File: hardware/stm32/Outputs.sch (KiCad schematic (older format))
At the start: 34 parts, among them J10 Screw_Terminal_01x02, J11 Screw_Terminal_01x02, J12 Screw_Terminal_01x02, J13 Screw_Terminal_01x02, J6 Screw_Terminal_01x02, J7 Conn_01x02, J8 Screw_Terminal_01x02, J9 Screw_Terminal_01x02, Q1 Q_NMOS_GSD, Q2 Q_NMOS_GSD, Q3 Q_NMOS_GSD, Q4 Q_NMOS_GSD, Q5 Q_NMOS_GSD, Q6 Q_NMOS_GSD, U10 PC817, U11 PC817, U5 PC817, U6 PC817, U7 PC817, U8 PC817, U9 PC817

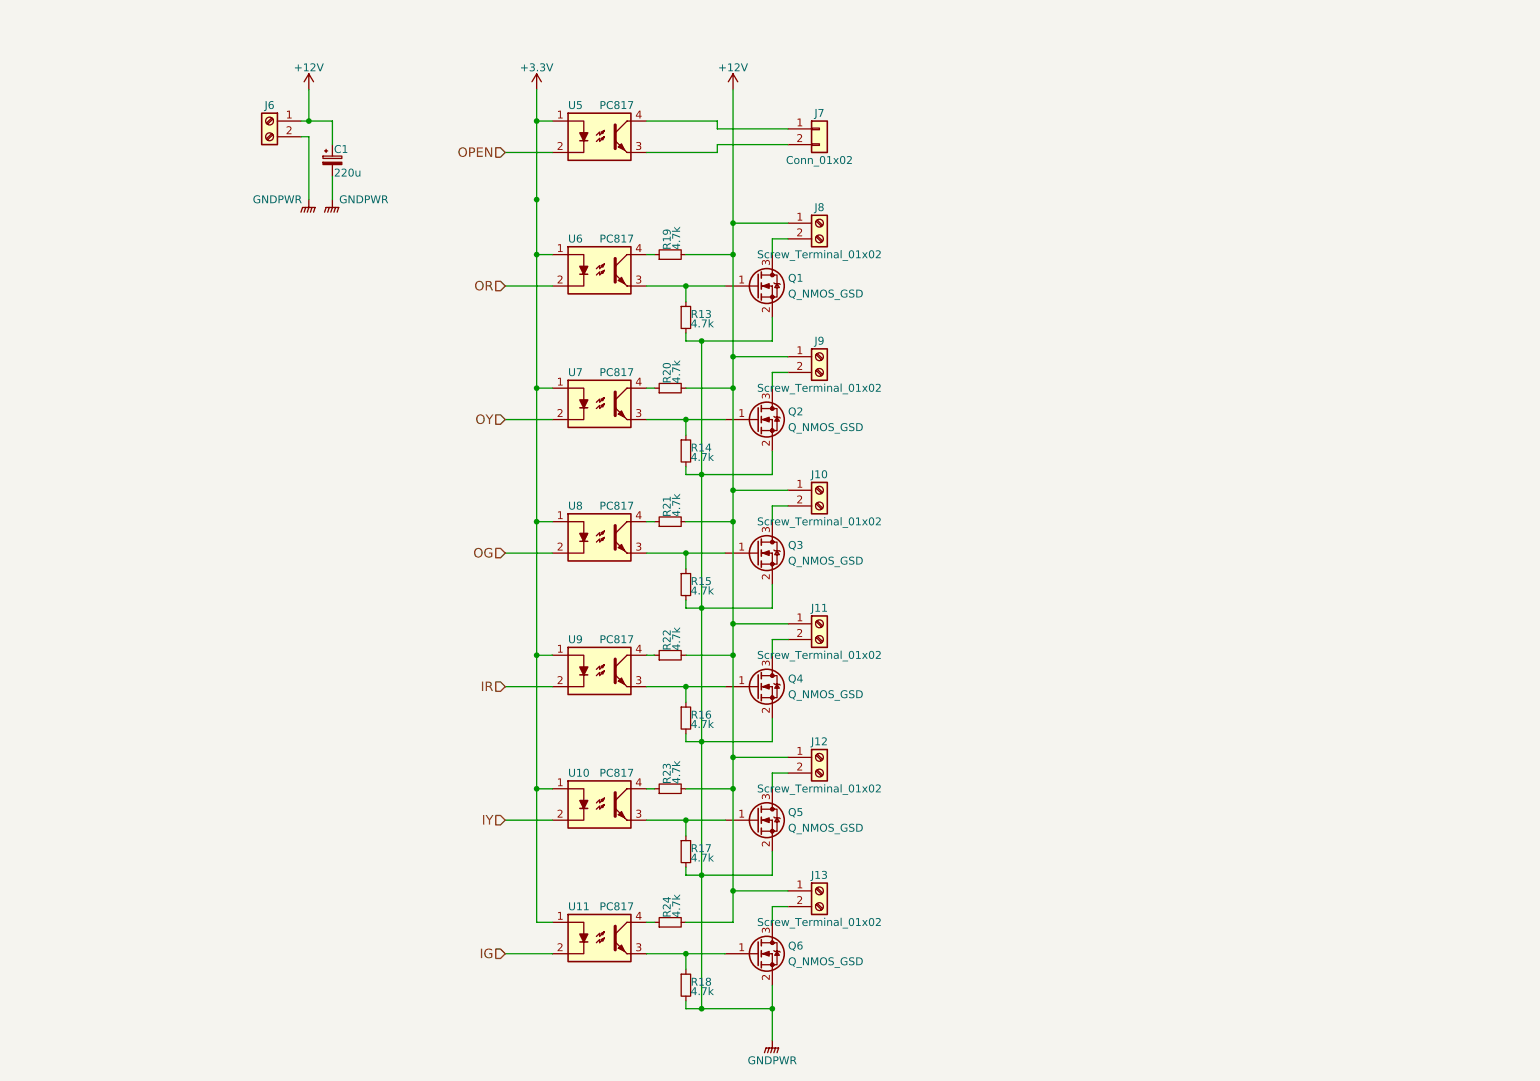
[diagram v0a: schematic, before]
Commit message: bluepill PCB progress
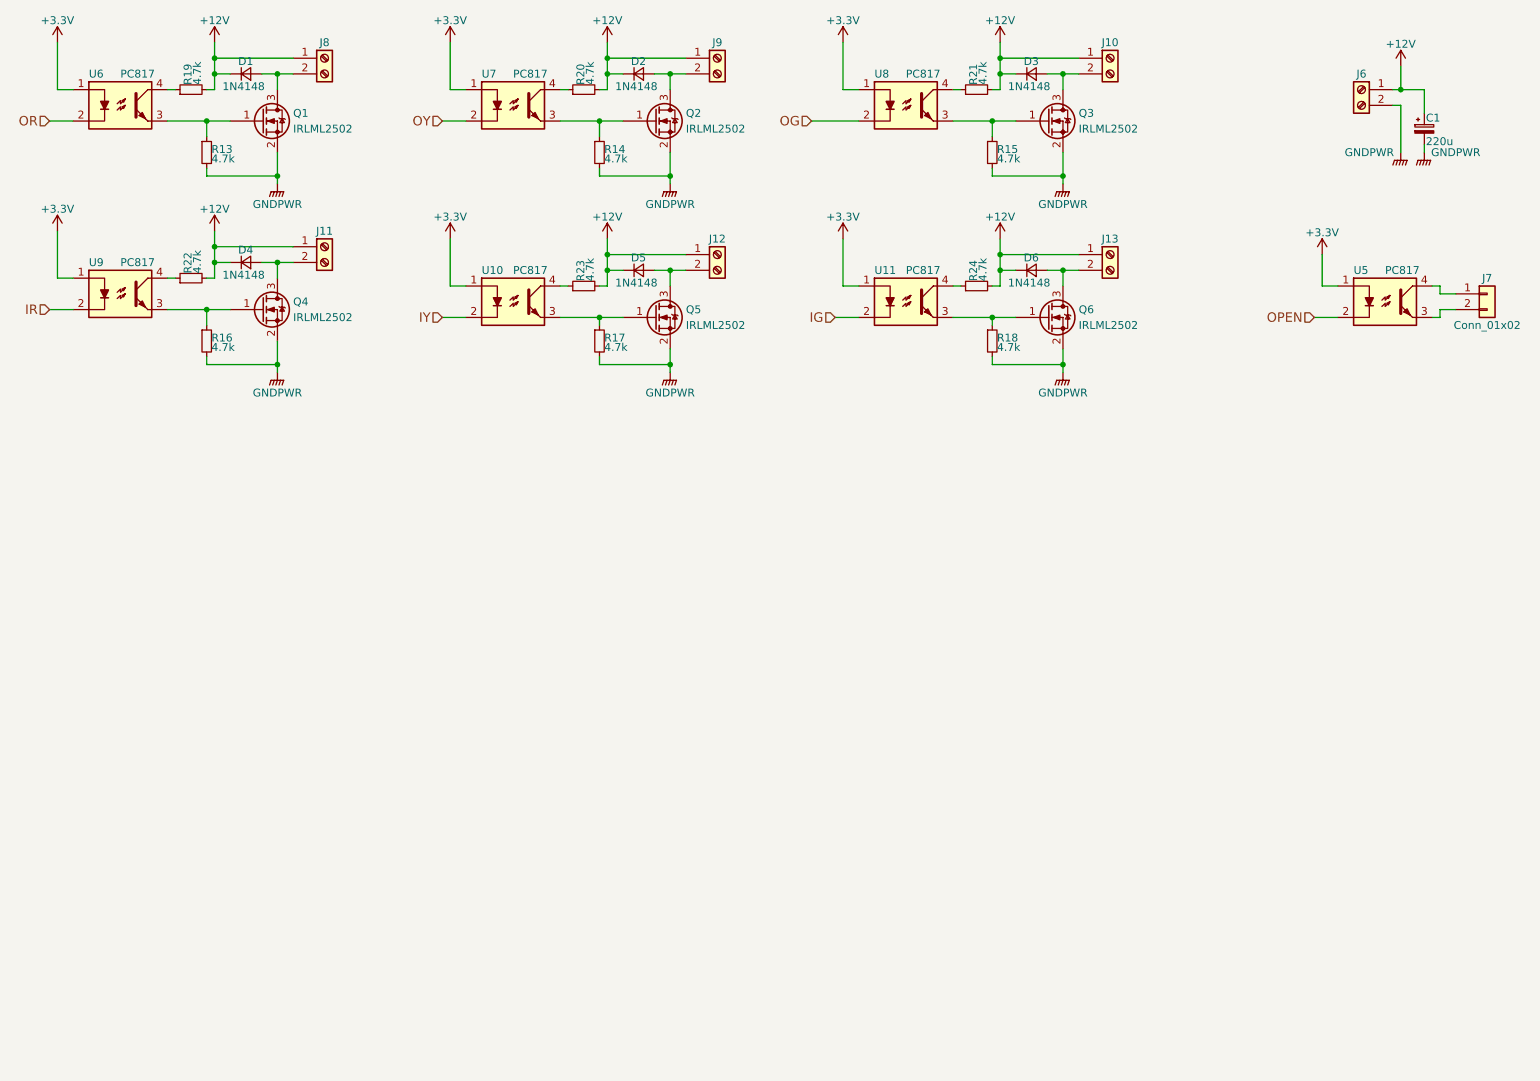
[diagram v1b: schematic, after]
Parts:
- added D1, D2, D3, D4, D5, D6: 1N4148, Diodes_SMD:D_MiniMELF, symbol D_Small
- Q1, Q2, Q3, Q4, Q5, Q6: value Q_NMOS_GSD -> IRLML2502
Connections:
- net +12V: now also D1.1 (K), D2.1 (K), D3.1 (K), D4.1 (K), D5.1 (K), D6.1 (K)
- net at J13.2 (Pin_2), Q6.3 (D): now also D6.2 (A)
- net at J12.2 (Pin_2), Q5.3 (D): now also D5.2 (A)
- net at J11.2 (Pin_2), Q4.3 (D): now also D4.2 (A)
- net at J10.2 (Pin_2), Q3.3 (D): now also D3.2 (A)
- net at J9.2 (Pin_2), Q2.3 (D): now also D2.2 (A)
- net at J8.2 (Pin_2), Q1.3 (D): now also D1.2 (A)
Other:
- moved on the sheet: C1, J10, J11, J12, J13, J6, J7, J8, J9, Q1, Q2, Q3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

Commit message: bluepill: PCB 0.9
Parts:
- U5: footprint Housings_DIP:DIP-4_W7.62mm -> Housings_DIP:DIP-4_W7.62mm_LongPads
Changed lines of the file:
@@
 F 0 "U5" H 9200 2700 50  0000 L CNN
 F 1 "PC817" H 9400 2700 50  0000 L CNN
-F 2 "Housings_DIP:DIP-4_W7.62mm" H 9200 2300 50  0001 L CIN
+F 2 "Housings_DIP:DIP-4_W7.62mm_LongPads" H 9200 2300 50  0001 L CIN
 F 3 "" H 9400 2500 50  0001 L CNN
 	1    9400 2500
@@
 $EndComp
 $Comp
-L +3.3V #PWR031
+L +3.3V #PWR46
 U 1 1 5A5FF7EF
 P 9000 2200
-F 0 "#PWR031" H 9000 2050 50  0001 C CNN
+F 0 "#PWR46" H 9000 2050 50  0001 C CNN
 F 1 "+3.3V" H 9000 2340 50  0000 C CNN
 F 2 "" H 9000 2200 50  0001 C CNN
@@
 $EndComp
 $Comp
-L +12V #PWR033
+L +12V #PWR47
 U 1 1 5A600289
 P 9500 1000
-F 0 "#PWR033" H 9500 850 50  0001 C CNN
+F 0 "#PWR47" H 9500 850 50  0001 C CNN
 F 1 "+12V" H 9500 1140 50  0000 C CNN
 F 2 "" H 9500 1000 50  0001 C CNN
@@
 $EndComp
 $Comp
-L GNDPWR #PWR034
+L GNDPWR #PWR45
 U 1 1 5A601D85
 P 7350 2950
-F 0 "#PWR034" H 7350 2750 50  0001 C CNN
+F 0 "#PWR45" H 7350 2750 50  0001 C CNN
 F 1 "GNDPWR" H 7350 2820 50  0000 C CNN
 F 2 "" H 7350 2900 50  0001 C CNN
@@
 $EndComp
 $Comp
-L GNDPWR #PWR035
+L GNDPWR #PWR49
 U 1 1 5A6021DD
 P 9650 1550
-F 0 "#PWR035" H 9650 1350 50  0001 C CNN
+F 0 "#PWR49" H 9650 1350 50  0001 C CNN
 F 1 "GNDPWR" H 9850 1550 50  0000 C CNN
 F 2 "" H 9650 1500 50  0001 C CNN
@@
 $EndComp
 $Comp
-L GNDPWR #PWR036
+L GNDPWR #PWR48
 U 1 1 5A6022C8
 P 9500 1550
-F 0 "#PWR036" H 9500 1350 50  0001 C CNN
+F 0 "#PWR48" H 9500 1350 50  0001 C CNN
 F 1 "GNDPWR" H 9300 1550 50  0000 C CNN
 F 2 "" H 9500 1500 50  0001 C CNN
@@
 $EndComp
 $Comp
-L +3.3V #PWR?
+L +3.3V #PWR41
 U 1 1 5A6240B1
 P 5950 2100
-F 0 "#PWR?" H 5950 1950 50  0001 C CNN
+F 0 "#PWR41" H 5950 1950 50  0001 C CNN
 F 1 "+3.3V" H 5950 2240 50  0000 C CNN
 F 2 "" H 5950 2100 50  0001 C CNN
@@
 $EndComp
 $Comp
-L +12V #PWR?
+L +12V #PWR43
 U 1 1 5A6249DA
 P 6950 2100
-F 0 "#PWR?" H 6950 1950 50  0001 C CNN
+F 0 "#PWR43" H 6950 1950 50  0001 C CNN
 F 1 "+12V" H 6950 2240 50  0000 C CNN
 F 2 "" H 6950 2100 50  0001 C CNN
@@
 Connection ~ 4850 2300
 $Comp
-L +3.3V #PWR?
+L +3.3V #PWR40
 U 1 1 5A628130
 P 5950 850
-F 0 "#PWR?" H 5950 700 50  0001 C CNN
+F 0 "#PWR40" H 5950 700 50  0001 C CNN
 F 1 "+3.3V" H 5950 990 50  0000 C CNN
 F 2 "" H 5950 850 50  0001 C CNN
@@
 $EndComp
 $Comp
-L +12V #PWR?
+L +12V #PWR42
 U 1 1 5A6281B3
 P 6950 850
-F 0 "#PWR?" H 6950 700 50  0001 C CNN
+F 0 "#PWR42" H 6950 700 50  0001 C CNN
 F 1 "+12V" H 6950 990 50  0000 C CNN
 F 2 "" H 6950 850 50  0001 C CNN
@@
 	5950 1150 5950 850
 $Comp
-L GNDPWR #PWR?
+L GNDPWR #PWR44
 U 1 1 5A628708
 P 7350 1750
-F 0 "#PWR?" H 7350 1550 50  0001 C CNN
+F 0 "#PWR44" H 7350 1550 50  0001 C CNN
 F 1 "GNDPWR" H 7350 1620 50  0000 C CNN
 F 2 "" H 7350 1700 50  0001 C CNN
@@
 $EndComp
 $Comp
-L GNDPWR #PWR?
+L GNDPWR #PWR38
 U 1 1 5A6287DB
 P 4850 1750
-F 0 "#PWR?" H 4850 1550 50  0001 C CNN
+F 0 "#PWR38" H 4850 1550 50  0001 C CNN
 F 1 "GNDPWR" H 4850 1620 50  0000 C CNN
 F 2 "" H 4850 1700 50  0001 C CNN
@@
 $EndComp
 $Comp
-L GNDPWR #PWR?
+L GNDPWR #PWR39
 U 1 1 5A628886
 P 4850 2950
-F 0 "#PWR?" H 4850 2750 50  0001 C CNN
+F 0 "#PWR39" H 4850 2750 50  0001 C CNN
 F 1 "GNDPWR" H 4850 2820 50  0000 C CNN
 F 2 "" H 4850 2900 50  0001 C CNN
@@
 $EndComp
 $Comp
-L GNDPWR #PWR?
+L GNDPWR #PWR32
 U 1 1 5A628909
 P 2350 1750
-F 0 "#PWR?" H 2350 1550 50  0001 C CNN
+F 0 "#PWR32" H 2350 1550 50  0001 C CNN
 F 1 "GNDPWR" H 2350 1620 50  0000 C CNN
 F 2 "" H 2350 1700 50  0001 C CNN
@@
 $EndComp
 $Comp
-L GNDPWR #PWR?
+L GNDPWR #PWR33
 U 1 1 5A62898C
 P 2350 2950
-F 0 "#PWR?" H 2350 2750 50  0001 C CNN
+F 0 "#PWR33" H 2350 2750 50  0001 C CNN
 F 1 "GNDPWR" H 2350 2820 50  0000 C CNN
 F 2 "" H 2350 2900 50  0001 C CNN
@@
 $EndComp
 $Comp
-L +3.3V #PWR?
+L +3.3V #PWR34
 U 1 1 5A628A0F
 P 3450 850
-F 0 "#PWR?" H 3450 700 50  0001 C CNN
+F 0 "#PWR34" H 3450 700 50  0001 C CNN
 F 1 "+3.3V" H 3450 990 50  0000 C CNN
 F 2 "" H 3450 850 50  0001 C CNN
@@
 $EndComp
 $Comp
-L +3.3V #PWR?
+L +3.3V #PWR35
 U 1 1 5A628A92
 P 3450 2100
-F 0 "#PWR?" H 3450 1950 50  0001 C CNN
+F 0 "#PWR35" H 3450 1950 50  0001 C CNN
 F 1 "+3.3V" H 3450 2240 50  0000 C CNN
 F 2 "" H 3450 2100 50  0001 C CNN
@@
 $EndComp
 $Comp
-L +12V #PWR?
+L +12V #PWR36
 U 1 1 5A628B15
 P 4450 850
-F 0 "#PWR?" H 4450 700 50  0001 C CNN
+F 0 "#PWR36" H 4450 700 50  0001 C CNN
 F 1 "+12V" H 4450 990 50  0000 C CNN
 F 2 "" H 4450 850 50  0001 C CNN
@@
 $EndComp
 $Comp
-L +12V #PWR?
+L +12V #PWR37
 U 1 1 5A628B98
 P 4450 2100
-F 0 "#PWR?" H 4450 1950 50  0001 C CNN
+F 0 "#PWR37" H 4450 1950 50  0001 C CNN
 F 1 "+12V" H 4450 2240 50  0000 C CNN
 F 2 "" H 4450 2100 50  0001 C CNN
@@
 Connection ~ 4850 2900
 $Comp
-L +12V #PWR?
+L +12V #PWR30
 U 1 1 5A629244
 P 1950 850
-F 0 "#PWR?" H 1950 700 50  0001 C CNN
+F 0 "#PWR30" H 1950 700 50  0001 C CNN
 F 1 "+12V" H 1950 990 50  0000 C CNN
 F 2 "" H 1950 850 50  0001 C CNN
@@
 $EndComp
 $Comp
-L +12V #PWR?
+L +12V #PWR31
 U 1 1 5A6292C7
 P 1950 2050
-F 0 "#PWR?" H 1950 1900 50  0001 C CNN
+F 0 "#PWR31" H 1950 1900 50  0001 C CNN
 F 1 "+12V" H 1950 2190 50  0000 C CNN
 F 2 "" H 1950 2050 50  0001 C CNN
@@
 $EndComp
 $Comp
-L +3.3V #PWR?
+L +3.3V #PWR28
 U 1 1 5A62934A
 P 950 850
-F 0 "#PWR?" H 950 700 50  0001 C CNN
+F 0 "#PWR28" H 950 700 50  0001 C CNN
 F 1 "+3.3V" H 950 990 50  0000 C CNN
 F 2 "" H 950 850 50  0001 C CNN
@@
 $EndComp
 $Comp
-L +3.3V #PWR?
+L +3.3V #PWR29
 U 1 1 5A6293CD
 P 950 2050
-F 0 "#PWR?" H 950 1900 50  0001 C CNN
+F 0 "#PWR29" H 950 1900 50  0001 C CNN
 F 1 "+3.3V" H 950 2190 50  0000 C CNN
 F 2 "" H 950 2050 50  0001 C CNN
